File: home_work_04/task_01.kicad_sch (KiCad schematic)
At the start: 5 parts, among them Q1 BC327-40, SW1 SW_Push

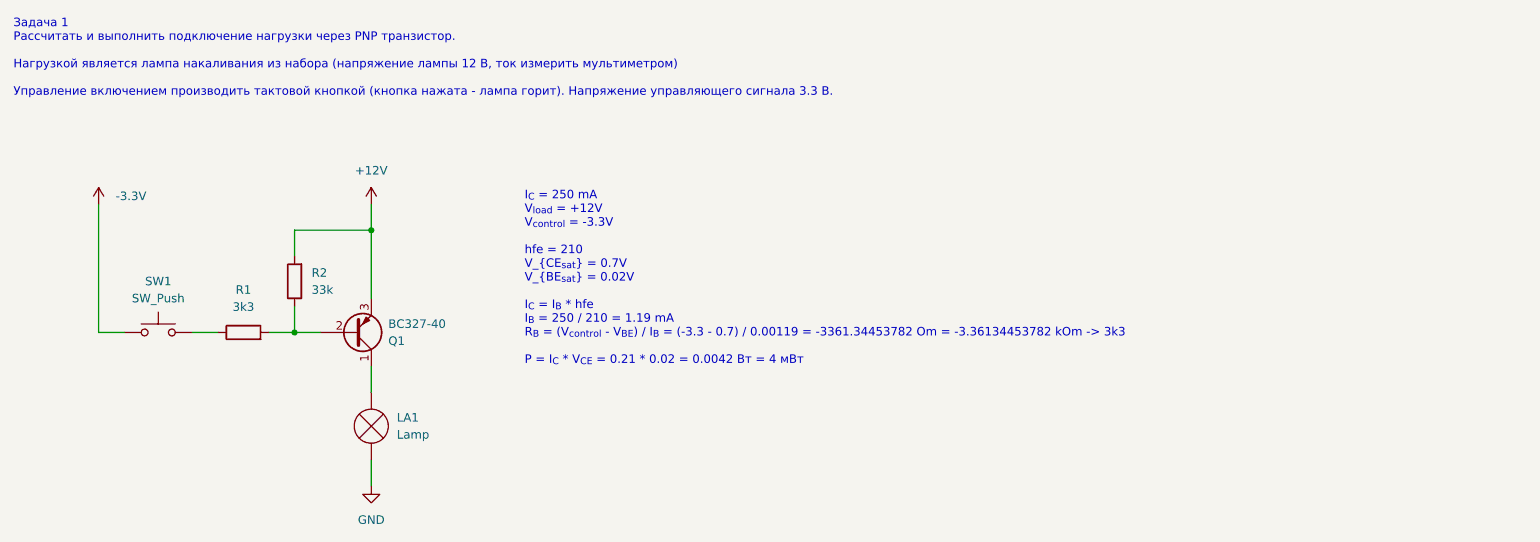
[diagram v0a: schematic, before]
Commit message: update home work 04
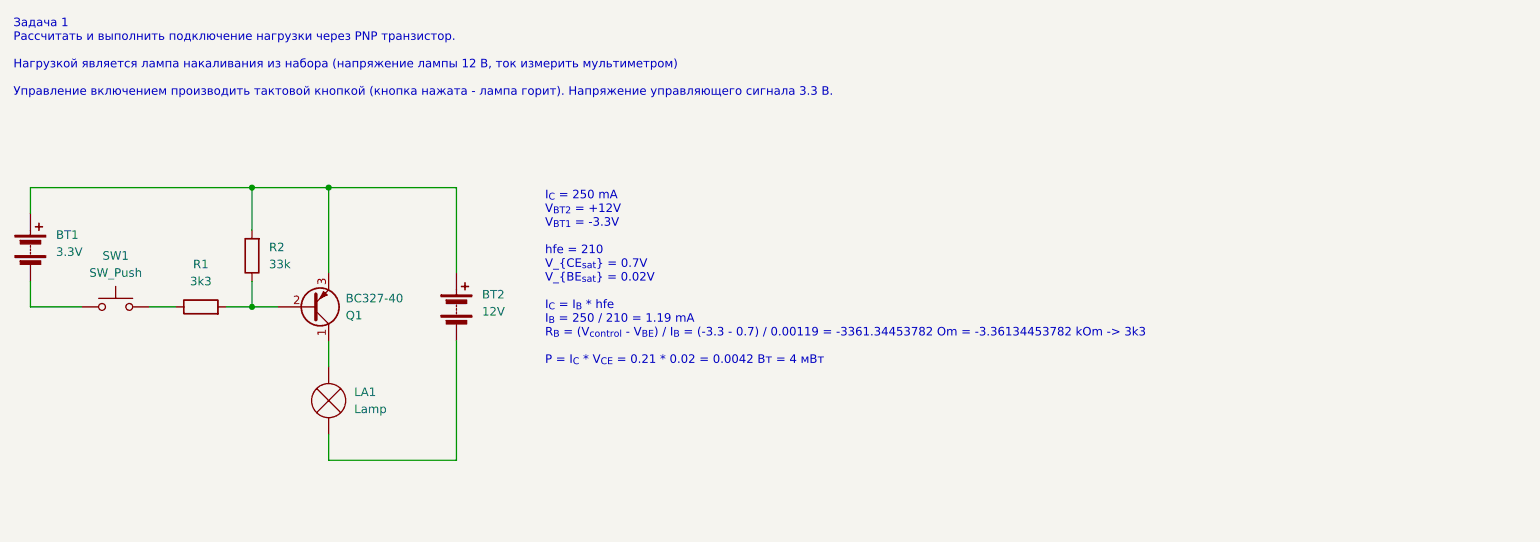
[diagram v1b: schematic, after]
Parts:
- added BT1: 3.3V, symbol Device:Battery
- added BT2: 12V, symbol Device:Battery
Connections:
- net +12V: no longer names the net of Q1.3 (E), R2.2
- net +12V: now also BT1.1 (+), BT2.1 (+)
- net -3.3V: no longer names the net of SW1.1
- net -3.3V: now also BT1.2 (-)
- net GND: no longer names the net of LA1.1 (-)
- net GND: now also BT2.2 (-)
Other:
- note added: "I_{C} = 250 mA V_{BT2} = +12V V_{BT1} = -3.3V hfe = 210 V_{CE_{sat}} = 0.7V V_{BE_{sat}} = 0.02V I_{C} = I_{B} * hfe I_{B} = 250 / 210 = 1.19 mA R_{B} = (V_{control} - V_{BE}) / I_{B} = (-3.3 - 0.7) / 0.00119 = -3361.34453782 Om = -3.36134453782 kOm -> 3k3 P = I_{C} * V_{CE} = 0.21 * 0.02 = 0.0042 Вт = 4 мВт"
- note removed: "I_{C} = 250 mA V_{load} = +12V V_{control} = -3.3V hfe = 210 V_{CE_{sat}} = 0.7V V_{BE_{sat}} = 0.02V I_{C} = I_{B} * hfe I_{B} = 250 / 210 = 1.19 mA R_{B} = (V_{control} - V_{BE}) / I_{B} = (-3.3 - 0.7) / 0.00119 = -3361.34453782 Om = -3.36134453782 kOm -> 3k3 P = I_{C} * V_{CE} = 0.21 * 0.02 = 0.0042 Вт = 4 мВт"
- moved on the sheet: LA1, Q1, R1, R2, SW1
